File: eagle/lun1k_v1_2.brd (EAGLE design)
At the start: 127.6 x 60.4 mm, 107 parts, among them IC1 LTC3558, IC2 LM27313, IC3 STM32F405RGT, IC4 NRF24L01SMD, J2 XF2-3015-1LW, Q1 Q12M-SMD-S, Q2 3.2X2.5CRYSTAL, SW1 JS102011SAQN, SW2 SWITCH_MCTAEF, SW3 SWITCH_MCTAEF, SW4 SWITCH_MCTAEF, U1 N35P112, X1 MICROUSB, X1_ JST-PH3

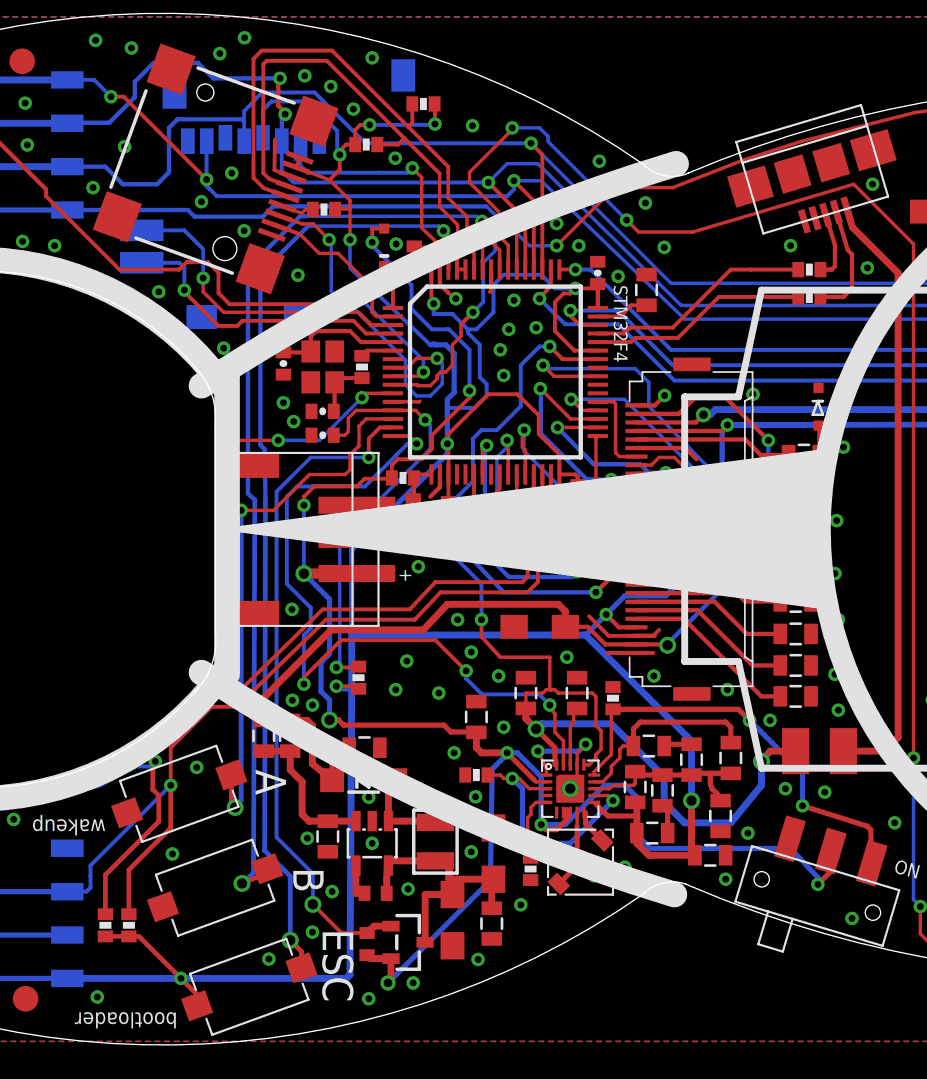
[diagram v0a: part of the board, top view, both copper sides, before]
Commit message: flash_db & adc & pcb misc
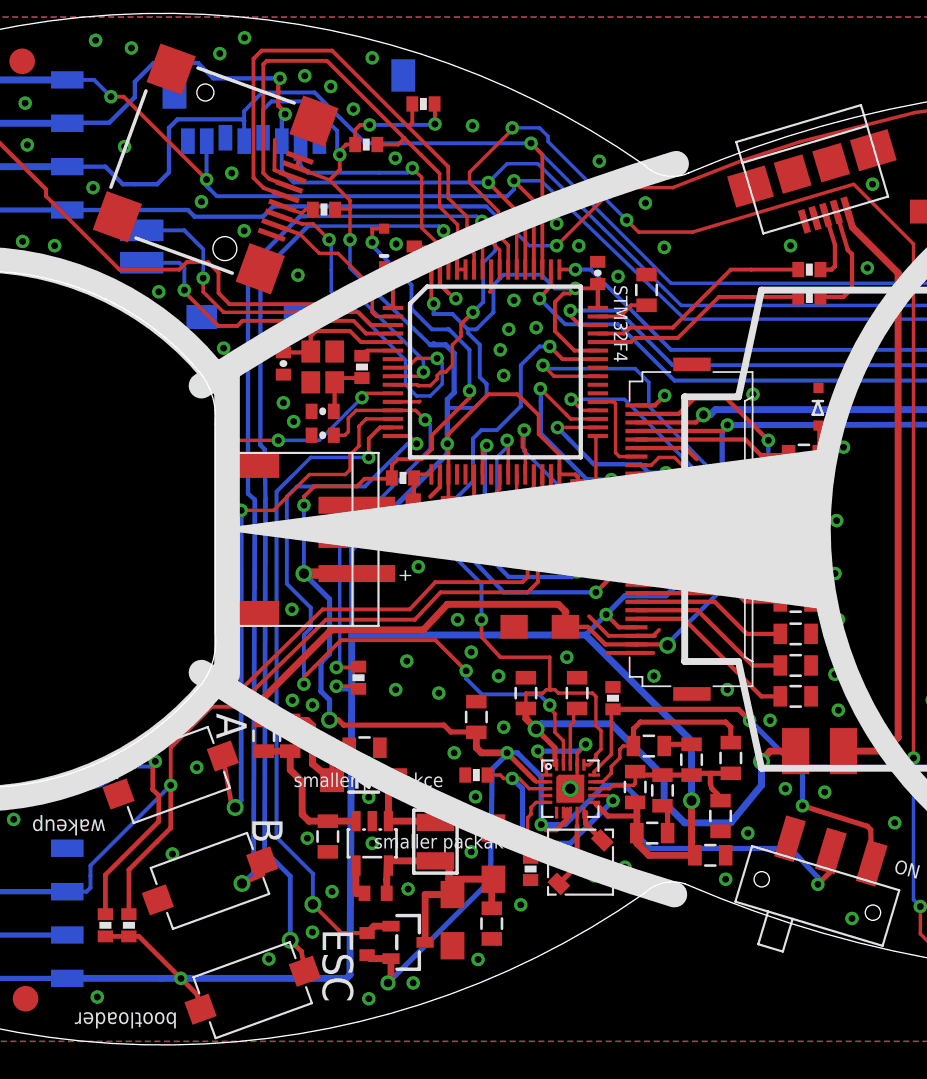
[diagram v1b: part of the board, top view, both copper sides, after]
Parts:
- moved SW4 1.21 mm to (-2.60, -14.4)
- moved SW3 0.50 mm to (-0.30, -20.6)
- moved SW2 0.28 mm to (2.20, -27.0)
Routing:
- net 3.3V: track 307.8 -> 306.9 mm
- net SW4: track 32.2 -> 33.0 mm
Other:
- board text added: "smaller packakce"
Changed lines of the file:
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@@
 <?xml version="1.0" encoding="utf-8"?>
 <!DOCTYPE eagle SYSTEM "eagle.dtd">
-<eagle version="6.2">
+<eagle version="6.6.0">
 <drawing>
 <settings>
@@
 <layer number="23" name="tOrigins" color="15" fill="1" visible="yes" active="yes"/>
 <layer number="24" name="bOrigins" color="15" fill="1" visible="no" active="yes"/>
-<layer number="25" name="tNames" color="7" fill="1" visible="no" active="yes"/>
+<layer number="25" name="tNames" color="7" fill="1" visible="yes" active="yes"/>
 <layer number="26" name="bNames" color="7" fill="1" visible="no" active="yes"/>
 <layer number="27" name="tValues" color="14" fill="1" visible="no" active="yes"/>
@@
 <wire x1="73.9" y1="13.34" x2="73.9" y2="-13.34" width="0.254" layer="21"/>
 <wire x1="47" y1="13.34" x2="47" y2="-13.34" width="0.254" layer="21"/>
-<text x="2.375" y="-14.075" size="1.778" layer="21" font="vector" rot="SR270">A</text>
-<text x="4.575" y="-19.8" size="1.778" layer="21" font="vector" rot="SR270">B</text>
+<text x="0.075" y="-10.775" size="1.778" layer="21" font="vector" rot="SR270">A</text>
+<text x="2.175" y="-16.9" size="1.778" layer="21" font="vector" rot="SR270">B</text>
 <text x="6.3" y="-23.4" size="1.778" layer="21" font="vector" rot="SR270">ESC</text>
 <text x="-6.4" y="-17" size="0.9" layer="21" font="vector" ratio="12" rot="SR180">wakeup</text>
@@
 <wire x1="35" y1="6.7" x2="35.6" y2="6.7" width="0.15" layer="21"/>
 <wire x1="35.6" y1="6.7" x2="35.3" y2="7.5" width="0.15" layer="21"/>
-<wire x1="35.3" y1="7.5" x2="35.6" y2="7.5" width="0.15" layer="21"/>
 <wire x1="35.6" y1="7.5" x2="35.3" y2="7.5" width="0.15" layer="21"/>
 <wire x1="35.3" y1="7.5" x2="35" y2="7.5" width="0.15" layer="21"/>
@@
 <text x="-16.375" y="27.575" size="1.2" layer="21" font="vector" ratio="12" rot="SR270">lun1k v1.2</text>
 <text x="-14.3" y="28.325" size="1.1" layer="21" font="vector" ratio="12" rot="SR270">seb@exse.net</text>
+<text x="9.3" y="-18.7" size="0.8128" layer="25">smaller packakce</text>
+<text x="4.6" y="-15.1" size="0.8128" layer="25">smaller packakce</text>
 </plain>
 <attributes>
@@
 </class>
 </classes>
-<designrules>
+<designrules name="default">
 <description language="de">&lt;b&gt;EAGLE Design Rules&lt;/b&gt;
 &lt;p&gt;
@@
 <attribute name="VALUE" x="11.2205" y="24.557" size="0.6096" layer="27" font="vector" ratio="12"/>
 </element>
-<element name="SW2" library="seb" package="SWITCH_MCTAEF" value="SWITCH_MCTAEF" x="2" y="-26.8" smashed="yes" rot="R200"/>
-<element name="SW3" library="seb" package="SWITCH_MCTAEF" value="SWITCH_MCTAEF" x="0" y="-21" smashed="yes" rot="R200"/>
-<element name="SW4" library="seb" package="SWITCH_MCTAEF" value="SWITCH_MCTAEF" x="-2.1" y="-15.5" smashed="yes" rot="R200"/>
+<element name="SW2" library="seb" package="SWITCH_MCTAEF" value="SWITCH_MCTAEF" x="2.2" y="-27" smashed="yes" rot="R200"/>
+<element name="SW3" library="seb" package="SWITCH_MCTAEF" value="SWITCH_MCTAEF" x="-0.3" y="-20.6" smashed="yes" rot="R200"/>
+<element name="SW4" library="seb" package="SWITCH_MCTAEF" value="SWITCH_MCTAEF" x="-2.6" y="-14.4" smashed="yes" rot="R200"/>
 <element name="IC1" library="seb" package="UD-QFN20" value="LTC3558" x="20.8" y="-15.2" smashed="yes">
 <attribute name="VALUE" x="18.46" y="-16.81" size="0.6096" layer="27" font="vector" ratio="12"/>
@@
 <wire x1="8" y1="-9.4" x2="8" y2="-6" width="0.4064" layer="16"/>
 <wire x1="8" y1="-6" x2="8" y2="-1.2" width="0.3048" layer="16"/>
-<wire x1="8" y1="-1.2" x2="12.35" y2="3.15" width="0.3048" layer="16"/>
+<wire x1="8" y1="-1.2" x2="13.6" y2="4.4" width="0.3048" layer="16"/>
 <contactref element="J2" pad="13"/>
 <contactref element="J2" pad="14"/>
-<wire x1="12.35" y1="3.15" x2="13.6" y2="4.4" width="0.3048" layer="16"/>
 <wire x1="13.6" y1="4.4" x2="13.6" y2="5" width="0.3048" layer="16"/>
 <wire x1="20.1644" y1="3.2062" x2="21.0938" y2="3.2062" width="0.2286" layer="1"/>
@@
 <wire x1="29.7" y1="5.7" x2="29.7" y2="-0.6" width="0.3048" layer="16"/>
 <wire x1="29.7" y1="-0.6" x2="27.5" y2="-2.8" width="0.3048" layer="16"/>
-<wire x1="27.5" y1="-2.8" x2="26.65" y2="-3.65" width="0.3048" layer="16"/>
-<wire x1="26.65" y1="-3.65" x2="26.4" y2="-3.9" width="0.3048" layer="16"/>
+<wire x1="27.5" y1="-2.8" x2="26.4" y2="-3.9" width="0.3048" layer="16"/>
 <wire x1="26.4" y1="-3.9" x2="24" y2="-3.9" width="0.3048" layer="16"/>
 <wire x1="24" y1="-3.9" x2="22.9" y2="-5" width="0.3048" layer="16"/>
-<wire x1="22.9" y1="-5" x2="22.75" y2="-5.15" width="0.3048" layer="16"/>
-<wire x1="22.75" y1="-5.15" x2="21.7" y2="-6.2" width="0.3048" layer="16"/>
+<wire x1="22.9" y1="-5" x2="21.7" y2="-6.2" width="0.3048" layer="16"/>
 <wire x1="21.7" y1="-6.2" x2="8.2" y2="-6.2" width="0.4064" layer="16"/>
 <wire x1="8.2" y1="-6.2" x2="8" y2="-6" width="0.3048" layer="16"/>
@@
 <wire x1="-2" y1="-26.31" x2="-3.15" y2="-26.31" width="0.4064" layer="16"/>
 <wire x1="-3.15" y1="-26.31" x2="-8.6565" y2="-26.31" width="0.4064" layer="16"/>
-<wire x1="-1.054" y1="-27.9115625" x2="-1.054" y2="-27.256" width="0.2794" layer="1"/>
+<wire x1="-0.854" y1="-28.1115625" x2="-1.054" y2="-27.256" width="0.2794" layer="1"/>
 <wire x1="-1.054" y1="-27.256" x2="-2" y2="-26.31" width="0.2794" layer="1"/>
 <via x="-2" y="-26.31" extent="1-16" drill="0.4"/>
-<wire x1="-2" y1="-26.31" x2="-3.15" y2="-26.31" width="0.2794" layer="16"/>
 <wire x1="-5.05" y1="-23.85" x2="-4.46" y2="-23.85" width="0.2794" layer="1"/>
 <wire x1="-4.46" y1="-23.85" x2="-2" y2="-26.31" width="0.2794" layer="1"/>
@@
 <wire x1="12.825" y1="23.675" x2="12.875" y2="23.725" width="0.2286" layer="16"/>
 <via x="12.875" y="23.725" extent="1-16" drill="0.4"/>
-<wire x1="12.875" y1="23.725" x2="12.875" y2="24.2" width="0.2286" layer="1"/>
-<wire x1="12.875" y1="24.2" x2="12.875" y2="24.875" width="0.2286" layer="1"/>
+<wire x1="12.875" y1="23.725" x2="12.875" y2="24.875" width="0.2286" layer="1"/>
 <wire x1="12.875" y1="24.875" x2="12.85" y2="24.9" width="0.2286" layer="1"/>
 <wire x1="7.3" y1="21.925" x2="7.3" y2="22.15" width="0.2286" layer="1"/>
@@
 <wire x1="8.6" y1="6.2" x2="8.8438" y2="6.4562" width="0.2032" layer="1"/>
 <wire x1="8.8438" y1="6.4562" x2="10.4144" y2="6.4562" width="0.2032" layer="1"/>
-<wire x1="0.954" y1="-14.388434375" x2="0.954" y2="-16.079" width="0.2794" layer="1"/>
+<wire x1="0.454" y1="-13.288434375" x2="0.954" y2="-16.079" width="0.2794" layer="1"/>
 <wire x1="0.954" y1="-16.079" x2="1.175" y2="-16.3" width="0.2794" layer="1"/>
 <via x="1.175" y="-16.3" extent="1-16" drill="0.6"/>
@@
 <wire x1="3.425" y1="1.1" x2="1.525" y2="1.1" width="0.2032" layer="1"/>
 <via x="1.525" y="1.1" extent="1-16" drill="0.4"/>
-<wire x1="1.525" y1="1.1" x2="1.525" y2="0.725" width="0.2032" layer="16"/>
 </signal>
 <signal name="SW2">
@@
 <wire x1="13.375" y1="17.475" x2="13.1" y2="17.75" width="0.2032" layer="16"/>
 <wire x1="13.1" y1="17.75" x2="5.45" y2="17.75" width="0.2032" layer="16"/>
-<wire x1="5.054" y1="-25.688434375" x2="5.054" y2="-24.729" width="0.2794" layer="1"/>
+<wire x1="5.254" y1="-25.888434375" x2="5.054" y2="-24.729" width="0.2794" layer="1"/>
 <wire x1="5.054" y1="-24.729" x2="4.4" y2="-24.075" width="0.2794" layer="1"/>
 <via x="4.4" y="-24.075" extent="1-16" drill="0.6"/>
@@
 <wire x1="15.625" y1="18.025" x2="15.325" y2="18.325" width="0.2032" layer="16"/>
 <wire x1="15.325" y1="18.325" x2="5.35" y2="18.325" width="0.2032" layer="16"/>
-<wire x1="3.054" y1="-19.888434375" x2="3.079" y2="-20.129" width="0.2794" layer="1"/>
-<wire x1="3.079" y1="-20.129" x2="1.575" y2="-20.75" width="0.2794" layer="1"/>
+<wire x1="2.754" y1="-19.488434375" x2="2.779" y2="-20.229" width="0.2794" layer="1"/>
+<wire x1="2.779" y1="-20.229" x2="1.575" y2="-20.75" width="0.2794" layer="1"/>
 <via x="1.575" y="-20.75" extent="1-16" drill="0.6"/>
 <wire x1="1.575" y1="-20.75" x2="1.8" y2="-20.575" width="0.2794" layer="16"/>

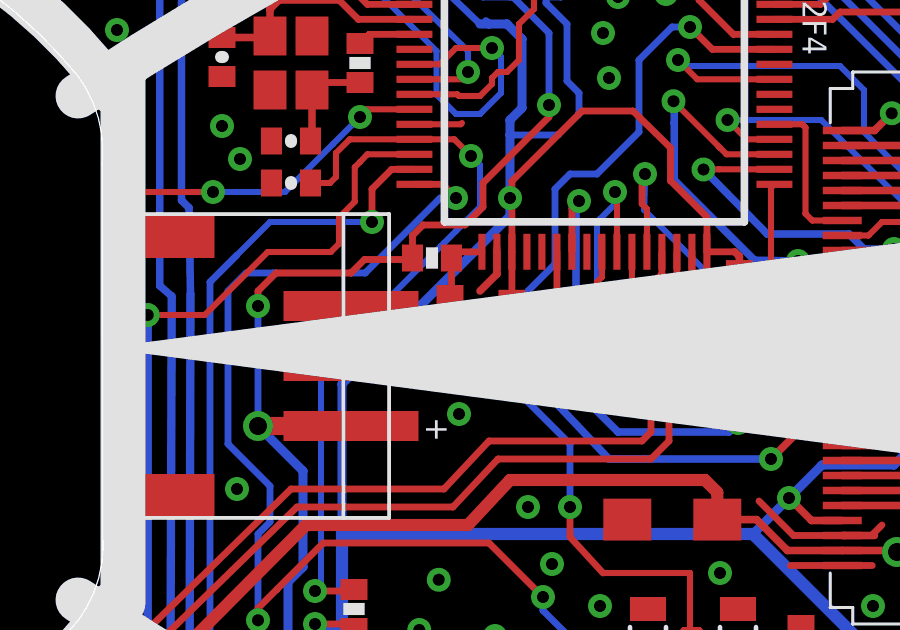
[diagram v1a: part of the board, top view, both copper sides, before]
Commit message: cap
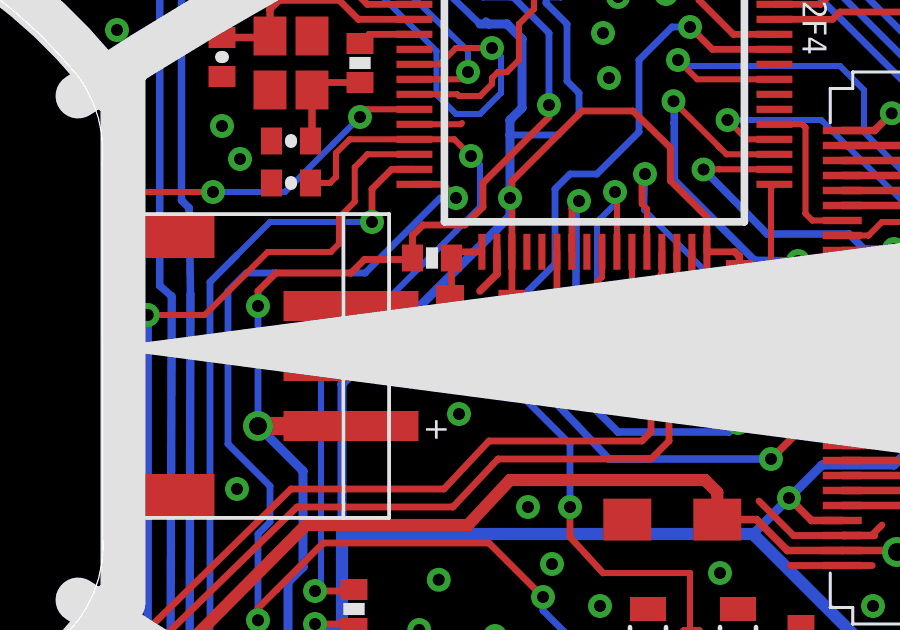
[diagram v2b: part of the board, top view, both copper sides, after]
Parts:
- added C27: 22pF, SparkFun-Capacitors:0402-CAP
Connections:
- net GND: now also C27.1
- net VOLTAGE: now also C27.2
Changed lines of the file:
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@@
 <attribute name="VALUE" x="6.995" y="-23.665" size="1.27" layer="27" rot="R270"/>
+</element>
+<element name="C27" library="SparkFun-Capacitors" package="0402-CAP" value="22pF" x="11.6" y="1.1" smashed="yes" rot="R90">
+<attribute name="VALUE" x="12.743" y="0.0205" size="0.4064" layer="27" rot="R90"/>
 </element>
 </elements>
@@
 <via x="5.7" y="-23.6" extent="1-16" drill="0.4"/>
 <via x="11.3" y="-21.075" extent="1-16" drill="0.4"/>
+<contactref element="C27" pad="1"/>
 </signal>
 <signal name="+5V" class="1">
@@
 <wire x1="11.65" y1="3" x2="11.65" y2="1.8" width="0.2286" layer="1"/>
 <wire x1="11.65" y1="1.8" x2="11.6" y2="1.75" width="0.2286" layer="1"/>
+<contactref element="C27" pad="2"/>
 </signal>
 <signal name="SCK">
